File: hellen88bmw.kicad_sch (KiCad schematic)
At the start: 303 parts, among them J1 USB_B_Mini, J14 VRIN1, J15 VRIN2, J16 VROUT1, J17 XH-8A, J18 AudioJack_THR, J19 MiniFit, J2 Conn_01x05, J20 ETB, J21 ETB, J4 Conn_01x05, M1 Module-power12-0.2, M10 Module-ign8-0.1, M11 Module-mcu144-0.5, M12 Module-knock-0.1, M13 Module-sd-0.1, M2 Module-can-0.1, M3 Module-wbo-0.2, M4 Module-can-0.1, M5 Module-power5-0.2, M6 Module-vr-0.1, M7 Module-input-0.1, M8 Module-knock-0.1, M9 Module-output-0.2, P1 P, P2 P, P3 P, P4 P, P5 P, P6 P, Q1 NGD8201AN, Q10 AUIPS2041LTR, Q2 NGD8201AN, Q3 NGD8201AN, Q4 NGD8201AN, Q5 NGD8201AN, Q6 NGD8201AN, Q7 NGD8201AN, Q8 NGD8201AN, Q9 AUIPS2041LTR, SW1 RESET, SW2 RESET, U1 MPXA6115A, U2 MPX4_MAP, U3 LIS2DW12TR, U4 LPS25HB, U5 MCP6002-xSN, U6 L6205PD

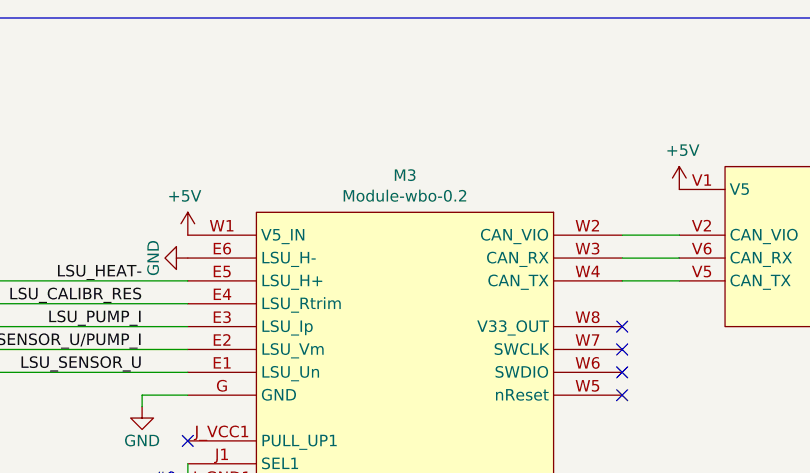
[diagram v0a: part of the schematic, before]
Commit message: Wbo 0.3
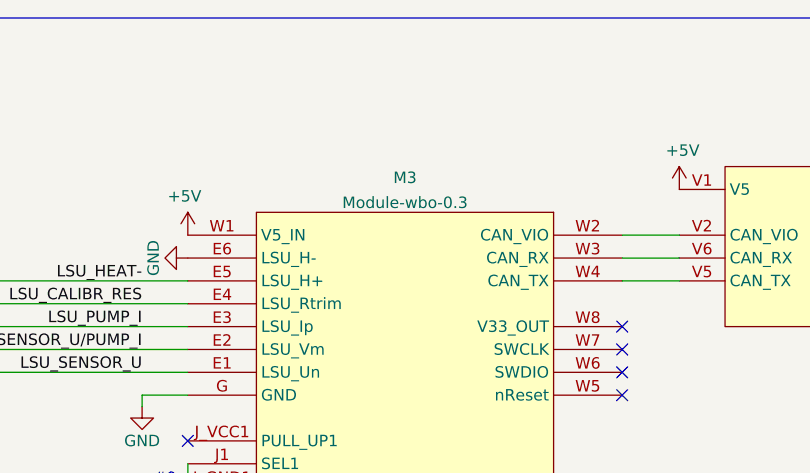
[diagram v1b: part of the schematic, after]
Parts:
- removed M3: Module-wbo-0.2, hellen-one-wbo-0.2:wbo, symbol hellen-one-wbo-0.2:Module-wbo-0.2
- added M3: Module-wbo-0.3, hellen-one-wbo-0.3:wbo, symbol hellen-one-wbo-0.3:Module-wbo-0.3
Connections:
- net +5V: now also M3.W1 (V5_IN)
- net GND: now also M3.E6 (LSU_H-), M3.G (GND)
- net LSU_CALIBR_RES: now also M3.E4 (LSU_Rtrim)
- net LSU_HEAT-: now also M3.E5 (LSU_H+)
- net LSU_PUMP_I: now also M3.E3 (LSU_Ip)
- net LSU_SENSOR_U: now also M3.E1 (LSU_Un)
- net LSU_SENSOR_U/PUMP_I: now also M3.E2 (LSU_Vm)
- net at M4.V2 (CAN_VIO): now also M3.W2 (CAN_VIO)
- net at M4.V6 (CAN_RX): now also M3.W3 (CAN_RX)
- net at M4.V5 (CAN_TX): now also M3.W4 (CAN_TX)
- new net: M3.J1 (SEL1), M3.J_GND1 (PULL_DOWN1)
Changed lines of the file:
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@@
     (pin "J9")
   )
-  (symbol (lib_id "hellen-one-wbo-0.2:Module-wbo-0.2") (at 711.2 45.72 0) (mirror y) (unit 1)
-    (in_bom yes) (on_board yes)
-    (property "Reference" "M3" (id 0) (at 694.69 41.6368 0))
-    (property "Value" "Module-wbo-0.2" (id 1) (at 694.69 43.9355 0))
-    (property "Footprint" "hellen-one-wbo-0.2:wbo" (id 2) (at 685.8 44.45 0)
+  (symbol (lib_id "hellen-one-wbo-0.3:Module-wbo-0.3") (at 711.2 45.72 0) (mirror y) (unit 1)
+    (in_bom yes) (on_board yes) (fields_autoplaced)
+    (property "Reference" "M3" (id 0) (at 694.69 41.8804 0))
+    (property "Value" "Module-wbo-0.3" (id 1) (at 694.69 44.6555 0))
+    (property "Footprint" "hellen-one-wbo-0.3:wbo" (id 2) (at 685.8 44.45 0)
       (effects (font (size 1.27 1.27)) hide)
     )
@@
       (reference "M2") (unit 1) (value "Module-can-0.1") (footprint "hellen-one-can-0.1:can")
     )
-    (path "/c145cecf-e6fb-4f01-91ef-f3fbeb476d3a"
-      (reference "M3") (unit 1) (value "Module-wbo-0.2") (footprint "hellen-one-wbo-0.2:wbo")
+    (path "/8f102ce2-a7ee-4380-a4d7-2d832c7c5a10"
+      (reference "M3") (unit 1) (value "Module-wbo-0.3") (footprint "hellen-one-wbo-0.3:wbo")
     )
     (path "/e3bc811d-dd8e-4541-8083-b187fedfc7e2"
